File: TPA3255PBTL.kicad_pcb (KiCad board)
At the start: 4 copper layers, 116 x 72 mm, 93 parts, among them J1 Barrel_Jack_Switch, J2 Conn_Coaxial, J3 Conn_02x04_Odd_Even, Q1 DMP4015SK3, Q2 DMN10H220L, Q3 DMN10H220L, SW1 SW_Push_Dual, U1 TPA3255DDV, U2 L78L12_SOT89, U3 L78L33_SO8, U4 NE5532, U5 XL7015

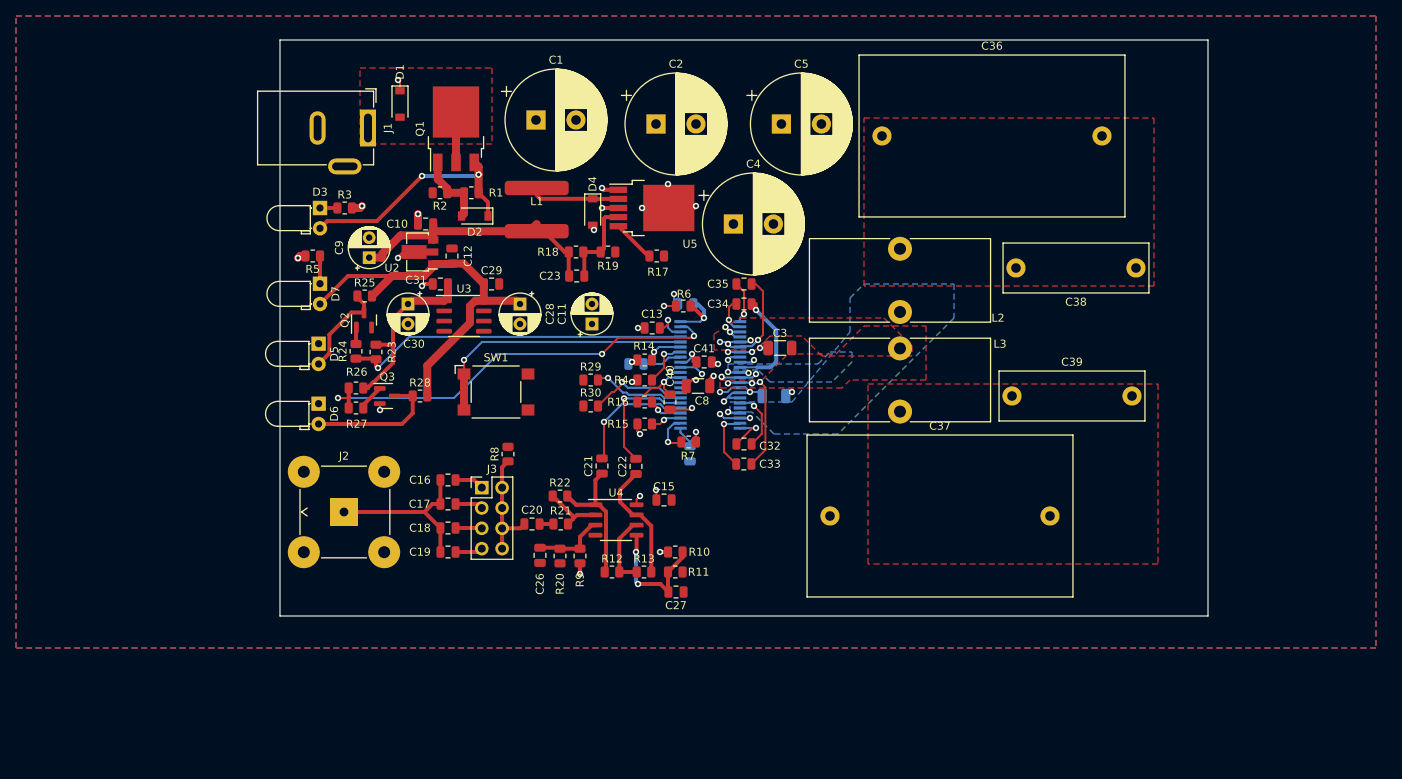
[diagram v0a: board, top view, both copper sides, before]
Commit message: Update, Post mfg
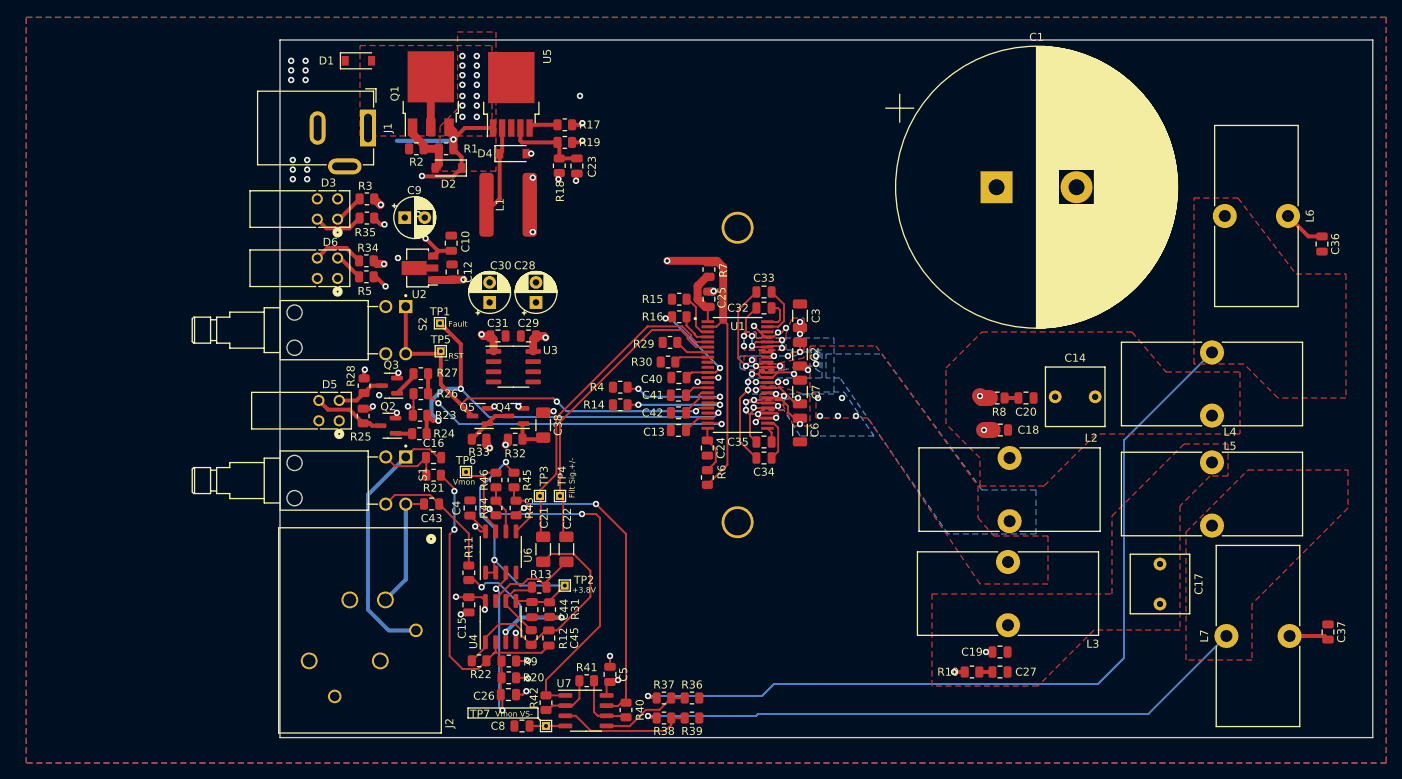
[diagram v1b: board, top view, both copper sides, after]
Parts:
- removed C11: 20u, Capacitor_THT:CP_Radial_D5.0mm_P2.50mm
- removed C39: 4.7n, Capacitor_THT:C_Rect_L18.0mm_W6.0mm_P15.00mm_FKS3_FKP3
- removed D7: LED, LED_THT:LED_D3.0mm_Horizontal_O1.27mm_Z2.0mm
- removed J3: Conn_02x04_Odd_Even, Connector_PinHeader_2.54mm:PinHeader_2x04_P2.54mm_Vertical
- removed SW1: SW_Push_Dual, Button_Switch_SMD:SW_SPST_Omron_B3FS-105xP
- added C14: 1u, Capacitor_THT:C_Rect_L7.2mm_W7.2mm_P5.00mm_FKS2_FKP2_MKS2_MKP2, F.Cu at (168.9, 88.6)
- added C43: 10n, Capacitor_SMD:C_0805_2012Metric, F.Cu at (91.0, 102.0)
- added C44: 330p, Capacitor_SMD:C_0805_2012Metric, F.Cu at (103.5, 115.2)
- added C45: 330p, Capacitor_SMD:C_0805_2012Metric, F.Cu at (105.6, 118.8)
- added L4: 10u, Inductor_THT:L_Toroid_Vertical_L22.4mm_W10.2mm_P7.90mm_Vishay_TJ4, F.Cu at (188.5, 91.0)
- added L5: 10u, Inductor_THT:L_Toroid_Vertical_L22.4mm_W10.2mm_P7.90mm_Vishay_TJ4, F.Cu at (188.5, 96.8)
- added L6: 10u, Inductor_THT:L_Toroid_Vertical_L22.4mm_W10.2mm_P7.90mm_Vishay_TJ4, F.Cu at (198.0, 66.0)
- added L7: 10u, Inductor_THT:L_Toroid_Vertical_L22.4mm_W10.2mm_P7.90mm_Vishay_TJ4, F.Cu at (190.3, 118.5)
- added Q4: DMN10H220L, Package_TO_SOT_SMD:SOT-23, F.Cu at (101.5, 91.0)
- added Q5: DMN10H220L, Package_TO_SOT_SMD:SOT-23, F.Cu at (97.0, 91.0)
- added R31: 10k, Resistor_SMD:R_0805_2012Metric, F.Cu at (105.7, 115.2)
- added R32: 47k, Resistor_SMD:R_0805_2012Metric, F.Cu at (101.4, 93.9)
- added R33: 47k, Resistor_SMD:R_0805_2012Metric, F.Cu at (96.9, 93.9)
- added R34: 470, Resistor_SMD:R_0805_2012Metric, F.Cu at (82.8, 71.6)
- added R35: 2.7k, Resistor_SMD:R_0805_2012Metric, F.Cu at (82.9, 66.3)
- added R36: 1k, Resistor_SMD:R_0805_2012Metric, F.Cu at (123.5, 126.2)
- added R37: 10k, Resistor_SMD:R_0805_2012Metric, F.Cu at (120.0, 126.2)
- added R38: 10k, Resistor_SMD:R_0805_2012Metric, F.Cu at (120.0, 128.8)
- added R39: 1k, Resistor_SMD:R_0805_2012Metric, F.Cu at (123.5, 128.8)
- added R40: 10k, Resistor_SMD:R_0805_2012Metric, F.Cu at (115.2, 127.8)
- added R41: DNP, Resistor_SMD:R_0805_2012Metric, F.Cu at (110.3, 124.1)
- added R42: 10k, Resistor_SMD:R_0805_2012Metric, F.Cu at (105.2, 126.8)
- added R43: 10k, Resistor_SMD:R_0805_2012Metric, F.Cu at (101.5, 102.5)
- added R44: 10k, Resistor_SMD:R_0805_2012Metric, F.Cu at (99.0, 102.5)
- added R45: 10k, Resistor_SMD:R_0805_2012Metric, F.Cu at (101.2, 99.0)
- added R46: 10k, Resistor_SMD:R_0805_2012Metric, F.Cu at (99.0, 99.0)
- added S1: PB400EEQX, Eli_Lib:SW_PB400EEQX, F.Cu at (87.7, 96.1)
- added S2: PB400OAQX, Eli_Lib:SW_PB400EEQX, F.Cu at (87.7, 77.3)
- added TP1: TestPoint, TestPoint:TestPoint_THTPad_1.0x1.0mm_Drill0.5mm, F.Cu at (92.0, 79.4)
- added TP2: TestPoint, TestPoint:TestPoint_THTPad_1.0x1.0mm_Drill0.5mm, F.Cu at (107.6, 112.2)
- added TP3: TestPoint, TestPoint:TestPoint_THTPad_1.0x1.0mm_Drill0.5mm, F.Cu at (104.5, 101.0)
- added TP4: TestPoint, TestPoint:TestPoint_THTPad_1.0x1.0mm_Drill0.5mm, F.Cu at (107.0, 101.0)
- added TP5: TestPoint, TestPoint:TestPoint_THTPad_1.0x1.0mm_Drill0.5mm, F.Cu at (92.1, 82.9)
- added TP6: TestPoint, TestPoint:TestPoint_THTPad_1.0x1.0mm_Drill0.5mm, F.Cu at (95.2, 98.0)
- added TP7: TestPoint, TestPoint:TestPoint_THTPad_1.0x1.0mm_Drill0.5mm, F.Cu at (105.2, 129.8)
- added U6: AD8512, Package_SO:SO-8_3.9x4.9mm_P1.27mm, F.Cu at (99.6, 108.0)
- added U7: AD8512, Package_SO:SO-8_3.9x4.9mm_P1.27mm, F.Cu at (110.2, 127.8)
- C1: value C_Polarized -> 4700u; footprint Capacitor_THT:CP_Radial_D12.5mm_P5.00mm -> Capacitor_THT:CP_Radial_D35.0mm_P10.00mm_SnapIn
- C16, C20, C27: value 100n -> 10n
- C17: value 10n -> 1u; footprint Capacitor_SMD:C_0805_2012Metric -> Capacitor_THT:C_Rect_L7.2mm_W7.2mm_P5.00mm_FKS2_FKP2_MKS2_MKP2
- C19: value 100p -> 1n
- C2: value C_Polarized -> 1u; footprint Capacitor_THT:CP_Radial_D12.5mm_P5.00mm -> Capacitor_SMD:C_1206_3216Metric
- C21, C22: value 1u -> 47u; footprint Capacitor_SMD:C_0805_2012Metric -> Capacitor_SMD:C_1206_3216Metric_Pad1.33x1.80mm_HandSolder
- C24, C25, U1: moved to F.Cu
- C3: value C -> 1u
- C36, C37: value 220n -> 12n; footprint Capacitor_THT:C_Rect_L33.0mm_W20.0mm_P27.50mm_MKS4 -> Capacitor_SMD:C_0805_2012Metric
- C38: value 4.7n -> 47u; footprint Capacitor_THT:C_Rect_L18.0mm_W6.0mm_P15.00mm_FKS3_FKP3 -> Capacitor_SMD:C_1206_3216Metric_Pad1.33x1.80mm_HandSolder
- C4, C5: value C_Polarized -> 100n; footprint Capacitor_THT:CP_Radial_D12.5mm_P5.00mm -> Capacitor_SMD:C_0805_2012Metric
- C42: value 100n -> 47n; moved to F.Cu
- C6, C7: value C -> 1u; moved to F.Cu
- C8: value C -> 100n; footprint Capacitor_SMD:C_1206_3216Metric -> Capacitor_SMD:C_0805_2012Metric
- D3, D5, D6: value LED -> LED_Dual_KAKA; footprint LED_THT:LED_D3.0mm_Horizontal_O1.27mm_Z2.0mm -> Eli_Lib:IC4_WP934EB_2GD_KNB
- J2: value Conn_Coaxial -> AC3FAH2-XLR; footprint Connector_Coaxial:BNC_TEConnectivity_1478035_Horizontal -> Eli_Lib:AC3FAH2-F-XLR
- R10, R8: value 10k -> 3R3
- R20: value 10k -> 4.7k
- R5: value 1k -> 2.7k
- U4: value NE5532 -> AD8512
- moved C17 89.3 mm to (182.0, 109.5), turned to -90 degrees
- moved C38 76.7 mm to (104.9, 92.1), turned to -90 degrees
- moved C5 72.1 mm to (113.2, 123.3), turned to -90 degrees
- moved C18 70.1 mm to (162.1, 92.8), turned to 180 degrees
- moved C19 70.1 mm to (162.0, 120.5)
- moved C37 63.9 mm to (203.0, 118.0), turned to -90 degrees
- moved C20 63.7 mm to (165.2, 88.8), turned to 180 degrees
- moved R8 61.6 mm to (161.7, 88.8), turned to 0 degrees
- moved C1 58.2 mm to (161.6, 62.4)
- moved C36 56.6 mm to (202.2, 69.5), turned to -90 degrees
- moved C4 48.4 mm to (95.8, 102.5), turned to 90 degrees
- moved C8 47.9 mm to (102.2, 129.8), turned to 0 degrees
- moved C27 41.7 mm to (162.0, 123.0), turned to 0 degrees
- moved R10 40.0 mm to (158.5, 123.0), turned to 180 degrees
- moved C2 33.9 mm to (137.0, 83.3), turned to -90 degrees
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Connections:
- net OUTC renamed OUTA
- C17 pad 1: Input -> GND
- C17 pad 2: Net-(C17-Pad2) -> OUTB2
- C18 pad 1: Input -> OUTA2
- C18 pad 2: Net-(C18-Pad2) -> GND
- C19 pad 1: Input -> GND
- C19 pad 2: Net-(C19-Pad2) -> OUTB2
- C20 pad 1: Net-(C20-Pad1) -> OUTA2
- C26 pad 2: Net-(U4-Pad3) -> Net-(C26-Pad2)
- C27 pad 1: GND -> Net-(C27-Pad1)
- C27 pad 2: Net-(R10-Pad2) -> OUTB2
- C36 pad 1: Load1 -> Net-(C36-Pad1)
- C37 pad 2: Load2 -> Net-(C37-Pad2)
- C38 pad 1: Load1 -> GND
- C38 pad 2: GND -> Net-(C38-Pad2)
- C4 pad 1: +48V -> +12V
- C5 pad 1: +48V -> GND
- C5 pad 2: GND -> +12V
- C8 pad 1: +48V -> GND
- C8 pad 2: GND -> Net-(U7-Pad4)
- J2 pad 1: Input -> GND
- J2 pad 2: GND -> Net-(C43-Pad1)
- L2 pad 2: Load1 -> OUTA2
- L3 pad 2: Load2 -> OUTB2
- Q2 pad 3: Net-(D5-Pad2) -> Net-(D5-Pad4)
- Q3 pad 3: Net-(D6-Pad2) -> Net-(D5-Pad2)
- R10 pad 1: +12V -> Net-(C27-Pad1)
- R10 pad 2: Net-(R10-Pad2) -> GND
- R11 pad 1: Net-(R10-Pad2) -> Net-(C43-Pad2)
- R11 pad 2: GND -> Net-(C44-Pad1)
- R20 pad 1: Net-(U4-Pad3) -> Net-(C26-Pad2)
- R21 pad 1: Net-(C20-Pad2) -> Net-(C16-Pad2)
- R25 pad 1: Net-(D5-Pad2) -> Net-(D5-Pad4)
- R28 pad 1: Net-(D6-Pad2) -> Net-(D5-Pad2)
- R5 pad 1: Net-(D7-Pad1) -> Net-(D6-Pad2)
- R5 pad 2: GND -> +12V
- R8 pad 1: Net-(C20-Pad1) -> GND
- R8 pad 2: GND -> Net-(C20-Pad2)
- R9 pad 2: Net-(U4-Pad3) -> Net-(C26-Pad2)
- U4 pad 3: Net-(U4-Pad3) -> Net-(C44-Pad1)
- U4 pad 5: Net-(R10-Pad2) -> +3V8
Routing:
- net Load1: track 0.00 -> 105.4 mm, vias 0 -> 1
- net Load2: track 0.00 -> 77.6 mm, vias 0 -> 1
- net Net-(R42-Pad1): track 0.00 -> 42.8 mm, vias 0 -> 2
- net Net-(R40-Pad2): track 0.00 -> 39.6 mm, vias 0 -> 2
- net +3V8: track 0.00 -> 36.3 mm, vias 0 -> 2
- net Net-(C45-Pad1): track 7.82 -> 39.4 mm, vias 0 -> 2
- net +15V: track 33.4 -> 7.40 mm, vias 0 -> 5
- net +3V3: track 22.4 -> 47.6 mm, vias 0 -> 3
- net FiltInA: track 15.3 -> 40.5 mm, vias 1 -> 0
- net Net-(C26-Pad2): track 0.00 -> 24.4 mm, vias 0 -> 2
- net FiltInB: track 15.5 -> 38.9 mm, vias 1 -> 0
- net Net-(C44-Pad1): track 0.00 -> 23.0 mm, vias 0 -> 3
- net RST_: track 34.2 -> 52.1 mm, vias 1 -> 2
- net Net-(R38-Pad1): track 0.00 -> 16.9 mm
- net Net-(C43-Pad2): track 0.00 -> 16.8 mm
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- added copper zone on In2.Cu, net +15V
- added copper zone on F.Cu, net +48V
- added copper zone on F.Cu, net OUTA
- added copper zone on F.Cu, net OUTA2
- added copper zone on B.Cu, net OUTB
- added copper zone on F.Cu, net OUTB2
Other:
- board size 116 x 72 mm -> 136.6 x 87.2 mm
- board text added: "+3.8V"
- board text added: "Fault"
- board text added: "Filt Sig.+/-"
- board text added: "Vmon"
- board text added: "Vmon VS-"
- board text added: "_RST"
